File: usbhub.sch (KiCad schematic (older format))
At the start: 19 parts, among them U3 USB2514B_Bi, Y1 X1E0000210129 24Mhz 12pF

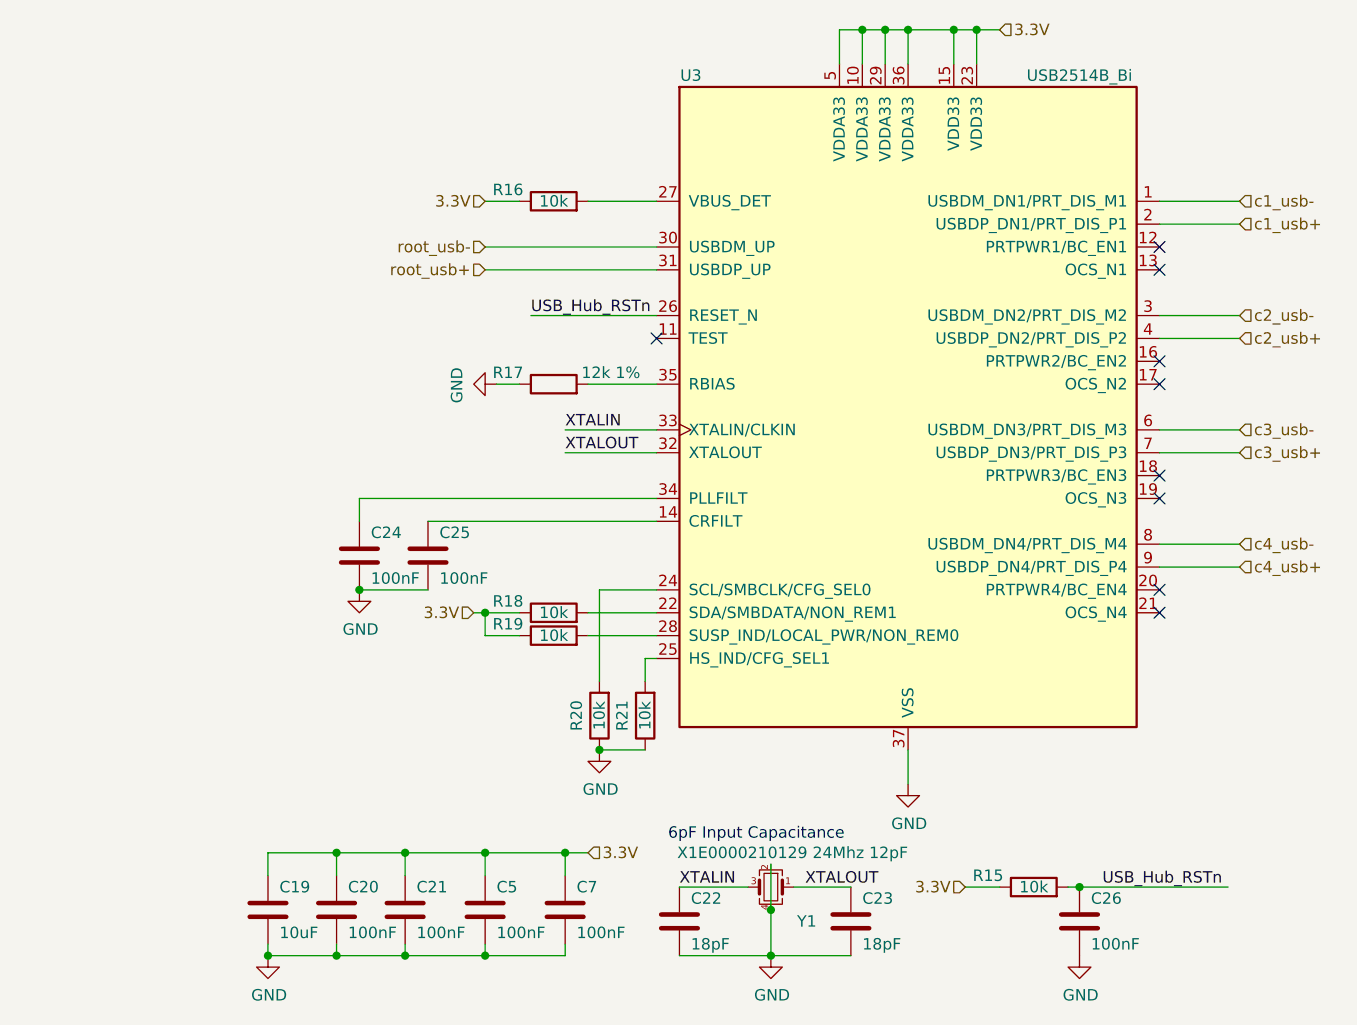
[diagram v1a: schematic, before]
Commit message: Changed USB Hub with Mux.
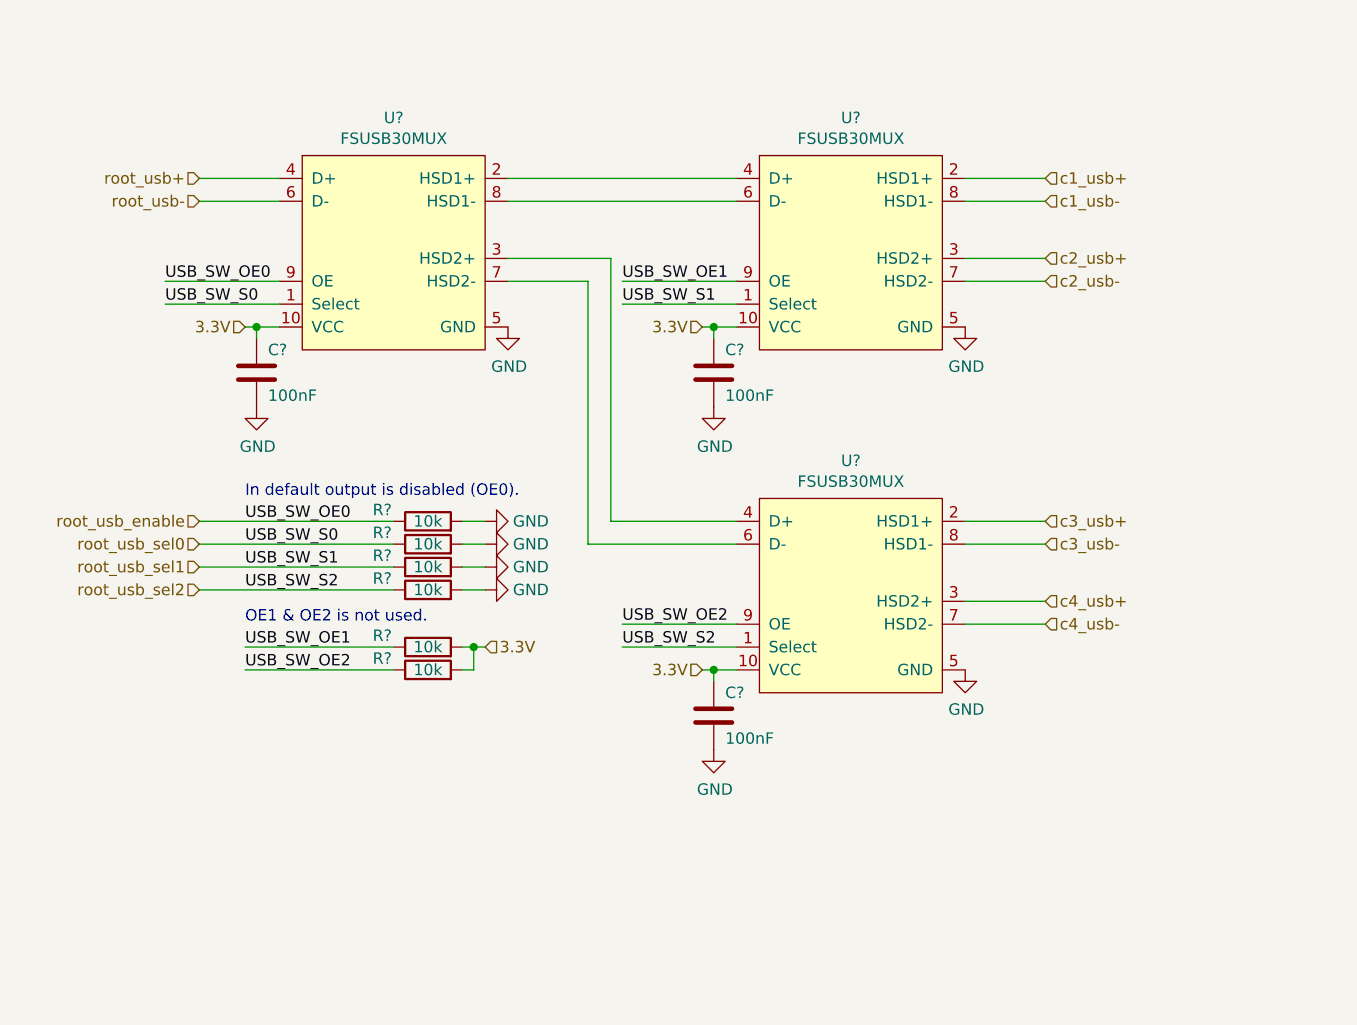
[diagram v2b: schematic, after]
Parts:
- removed C19: 10uF, Capacitor_SMD:C_0805_2012Metric, symbol Device:C
- removed C20, C21, C24, C25, C26, C5, C7: 100nF, Capacitor_SMD:C_0402_1005Metric, symbol Device:C
- removed C22, C23: 18pF, Capacitor_SMD:C_0402_1005Metric, symbol Device:C
- removed R15, R16, R18, R19, R20, R21: 10k, Resistor_SMD:R_0402_1005Metric, symbol Device:R
- removed R17: 12k 1%, Resistor_SMD:R_0402_1005Metric, symbol Device:R
- removed U3: USB2514B_Bi, Package_DFN_QFN:QFN-36-1EP_6x6mm_P0.5mm_EP3.7x3.7mm, symbol Interface_USB:USB2514B_Bi
- removed Y1: X1E0000210129 24Mhz 12pF, Crystal:Crystal_SMD_SeikoEpson_TSX3225-4Pin_3.2x2.5mm, symbol Device:Crystal_GND24_Small
- added C? (x3): 100nF, Capacitor_SMD:C_0402_1005Metric, symbol Device:C
- added R? (x6): 10k, Resistor_SMD:R_0402_1005Metric, symbol Device:R
- added U? (x3): FSUSB30MUX, Package_SO:MSOP-10_3x3mm_P0.5mm, symbol dg_ic:FSUSB30MUX
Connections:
- net 3.3V: now also C?.1, C?.1, C?.1, R?.2, R?.2, U?.10 (VCC), U?.10 (VCC), U?.10 (VCC)
- net GND: now also C?.2, C?.2, C?.2, R?.2, R?.2, R?.2, R?.2, U?.5 (GND), U?.5 (GND), U?.5 (GND)
- net c1_usb+: now also U?.2 (HSD1+)
- net c1_usb-: now also U?.8 (HSD1-)
- net c2_usb+: now also U?.3 (HSD2+)
- net c2_usb-: now also U?.7 (HSD2-)
- net c3_usb+: now also U?.2 (HSD1+)
- net c3_usb-: now also U?.8 (HSD1-)
- net c4_usb+: now also U?.3 (HSD2+)
- net c4_usb-: now also U?.7 (HSD2-)
- net root_usb+: now also U?.4 (D+)
- net root_usb-: now also U?.6 (D-)
- new net: U?.2 (HSD1+), U?.4 (D+)
- new net: U?.6 (D-), U?.8 (HSD1-)
- new net: U?.3 (HSD2+), U?.4 (D+)
- new net: U?.6 (D-), U?.7 (HSD2-)
- new net USB_SW_OE1: R?.1, U?.9 (OE)
- new net USB_SW_OE2: R?.1, U?.9 (OE)
- new net root_usb_enable: R?.1, U?.9 (OE)
- new net root_usb_sel0: R?.1, U?.1 (Select)
- new net root_usb_sel1: R?.1, U?.1 (Select)
- new net root_usb_sel2: R?.1, U?.1 (Select)
- no-connect marks 9 -> 0
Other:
- note added: "In default output is disabled (OE0)."
- note added: "OE1 & OE2 is not used."
- note removed: "6pF Input Capacitance"
